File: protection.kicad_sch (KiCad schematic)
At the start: 43 parts, among them K1 Relay_SPDT, Q1 BSS138, Q2 BSS138, SW1 SW_Push, U10 ADR4525, U11 74LVC1G32, U3 74LVC1G10, U4 LM339, U5 74LVC1G02, U6 74LVC1G32, U7 74LVC1G02, U8 74LVC1G02, U9 TPS3823-33DBV

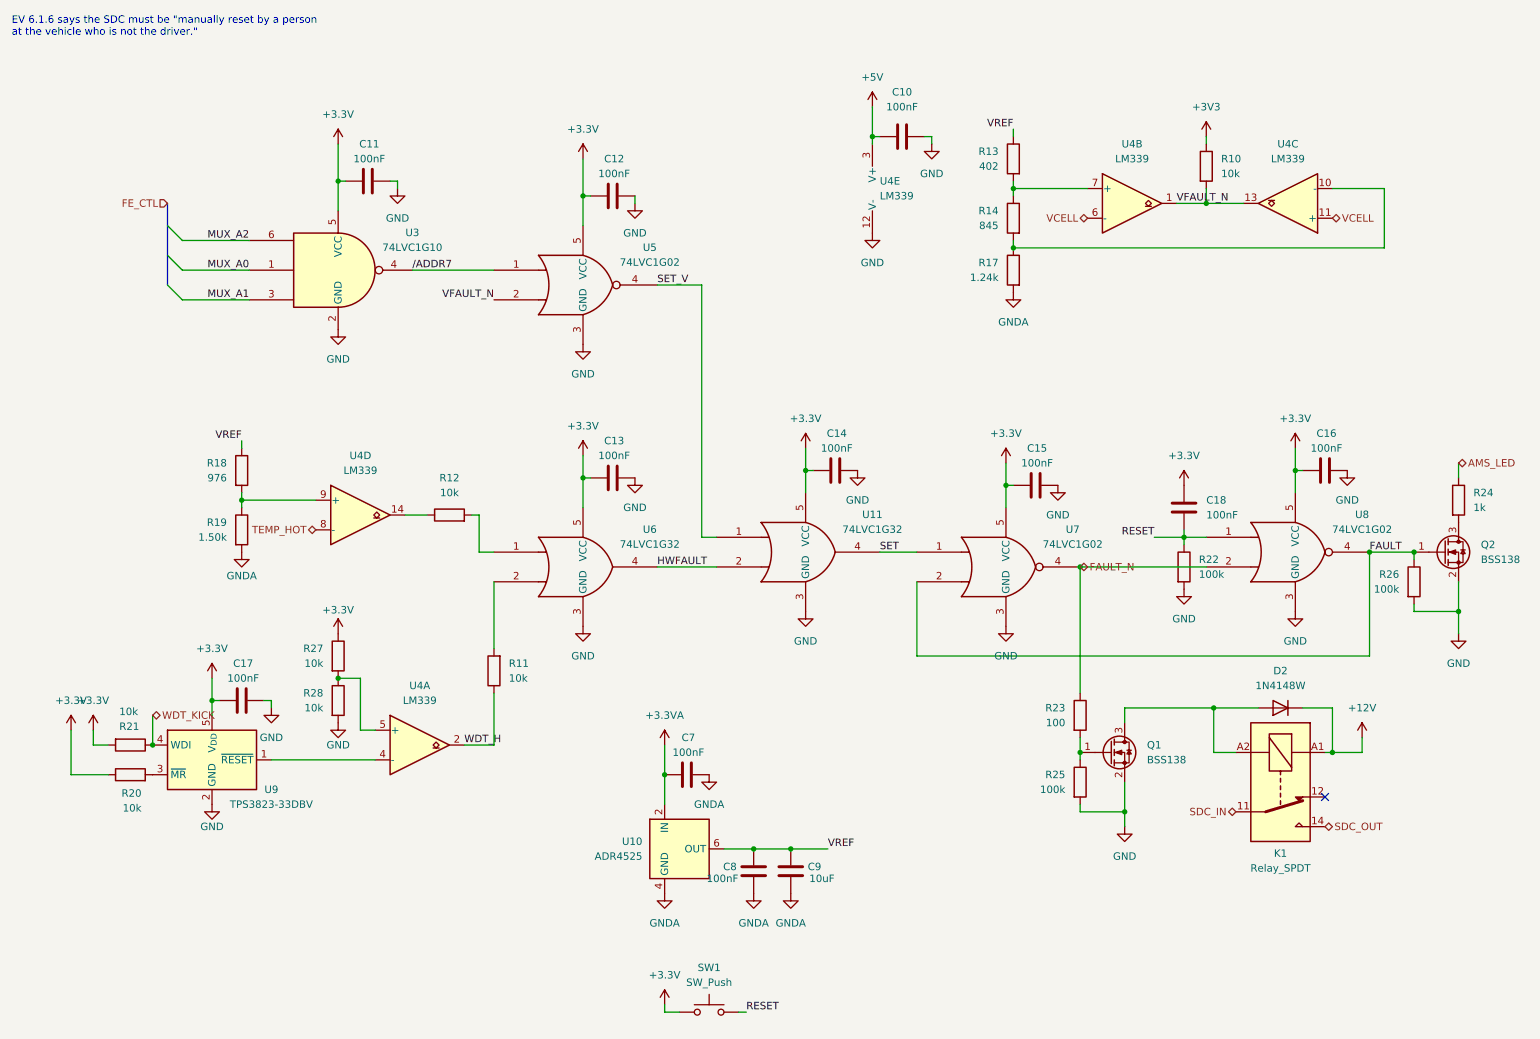
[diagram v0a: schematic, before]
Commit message: can transceiver; power; mcu
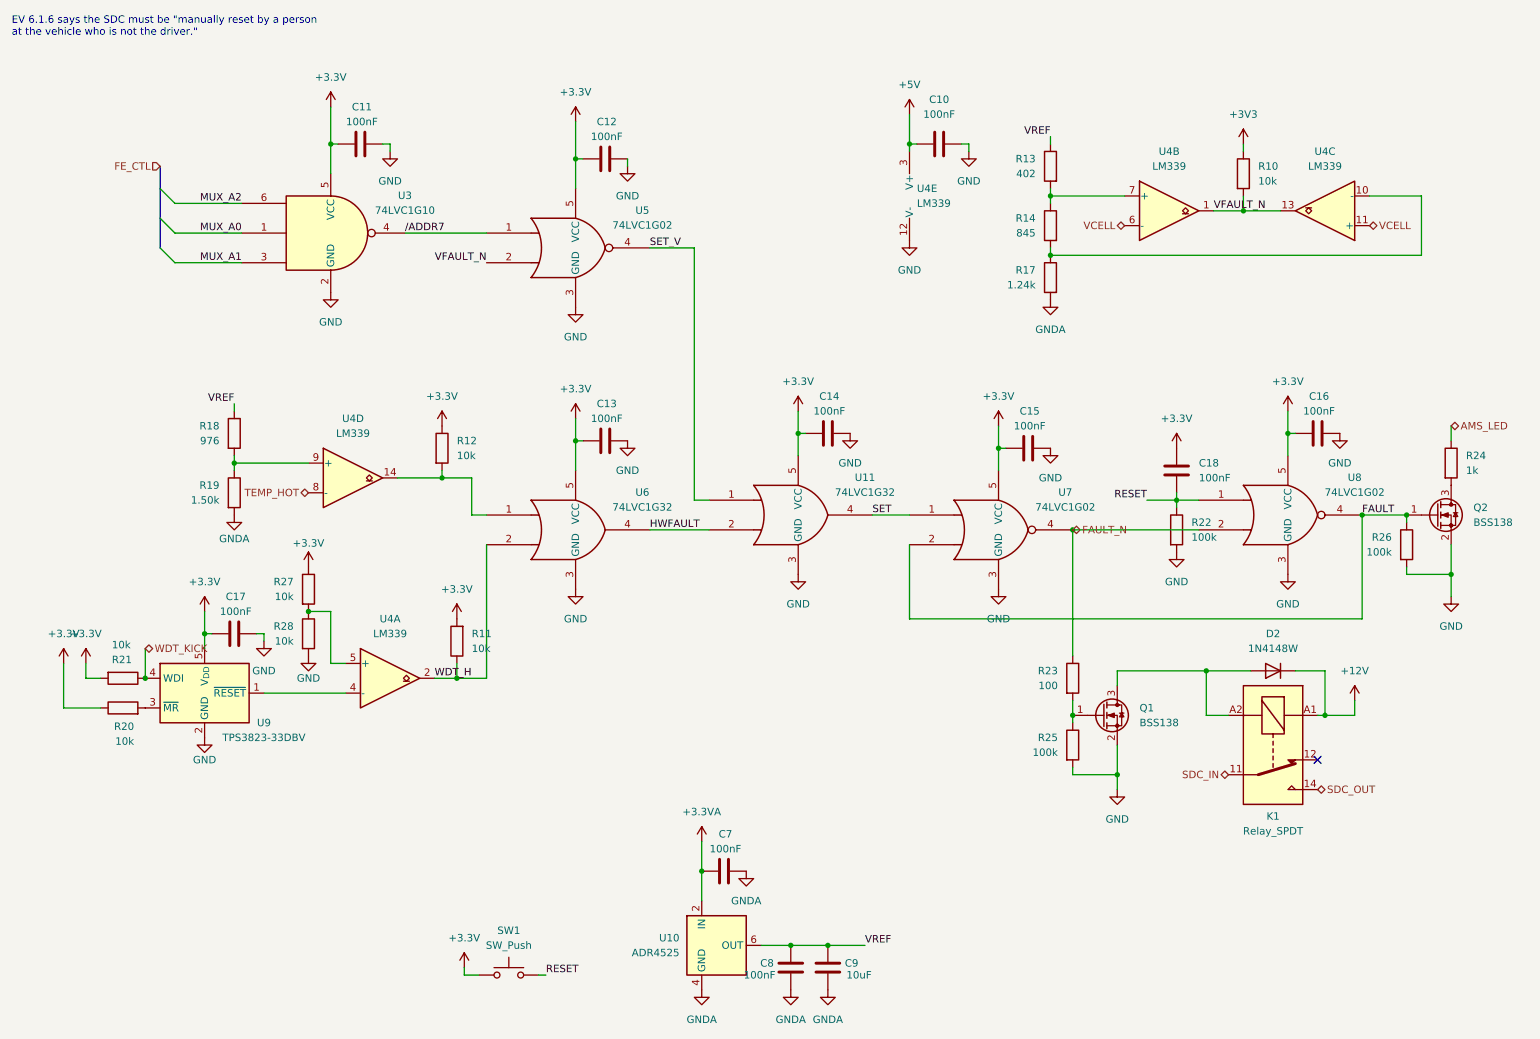
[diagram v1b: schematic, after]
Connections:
- net +3.3V: now also R11.2, R12.1
- net WDT_H: now also U6.2
- net at U4.14: now also R12.2, U6.1; no longer R12.1
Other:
- moved on the sheet: C10, C11, C12, C13, C14, C15, C16, C17, C18, C7, C8, C9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
